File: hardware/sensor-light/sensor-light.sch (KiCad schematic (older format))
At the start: 15 parts, among them J1 Power IN 12V, J2 PIR Sensor Header 2, J3 PIR Sensor Header 1, J4 PROG Header, J5 Light Sensor Header, J6 PWM Power OUT 12V, Q1 IRLML2502, SW1 Manual ON/OFF, U1 Reg 3.3V, U2 MSP430G2553IN20

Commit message: change lables on the schematic
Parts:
- J2: value PIR Sensor Header 2 -> PIR Sensor 2
- J3: value PIR Sensor Header 1 -> PIR Sensor 1
- J5: value Light Sensor Header -> Light Sensor
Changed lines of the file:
@@
 P 9650 4850
 F 0 "R2" V 9730 4850 50  0000 C CNN
-F 1 "100 KOhm" V 9650 4850 50  0000 C CNN
+F 1 "100 KOhm" V 9650 4850 50  0000 C BNN
 F 2 "" V 9580 4850 50  0001 C CNN
 F 3 "" H 9650 4850 50  0001 C CNN
@@
 P 9300 4200
 F 0 "R1" V 9380 4200 50  0000 C CNN
-F 1 "27 Ohm" V 9300 4200 50  0000 C CNN
+F 1 "27 Ohm" V 9300 4200 50  0000 C BNN
 F 2 "" V 9230 4200 50  0001 C CNN
 F 3 "" H 9300 4200 50  0001 C CNN
@@
 P 8950 3500
 F 0 "J5" H 8950 3775 50  0000 C CNN
-F 1 "Light Sensor Header" H 8975 3225 50  0000 C CNN
+F 1 "Light Sensor" H 8975 3225 50  0000 C CNN
 F 2 "" H 8950 3700 50  0001 C CNN
 F 3 "" H 8950 3700 50  0001 C CNN
@@
 P 3150 3950
 F 0 "J3" H 3150 4225 50  0000 C CNN
-F 1 "PIR Sensor Header 1" H 3175 3675 50  0000 C CNN
+F 1 "PIR Sensor 1" H 3175 3675 50  0000 C CNN
 F 2 "" H 3150 4150 50  0001 C CNN
 F 3 "" H 3150 4150 50  0001 C CNN
@@
 P 2550 4800
 F 0 "J2" H 2550 5075 50  0000 C CNN
-F 1 "PIR Sensor Header 2" H 2575 4525 50  0000 C CNN
+F 1 "PIR Sensor 2" H 2575 4525 50  0000 C CNN
 F 2 "" H 2550 5000 50  0001 C CNN
 F 3 "" H 2550 5000 50  0001 C CNN

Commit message: remove extra line on the schematics
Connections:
- wire segments 47 -> 62
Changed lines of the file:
@@
 $EndComp
 Wire Wire Line
-	1400 5500 9950 5500
+	1400 5500 1800 5500
+Wire Wire Line
+	1800 5500 2200 5500
+Wire Wire Line
+	2200 5500 2850 5500
+Wire Wire Line
+	2850 5500 3450 5500
+Wire Wire Line
+	3450 5500 3800 5500
+Wire Wire Line
+	3800 5500 5750 5500
+Wire Wire Line
+	5750 5500 7550 5500
+Wire Wire Line
+	7550 5500 7800 5500
+Wire Wire Line
+	7800 5500 8200 5500
+Wire Wire Line
+	8200 5500 8650 5500
+Wire Wire Line
+	8650 5500 9650 5500
+Wire Wire Line
+	9650 5500 9950 5500
 Wire Wire Line
 	5750 4950 5750 5500
 Wire Wire Line
-	2200 3300 8650 3300
+	2200 3300 2850 3300
+Wire Wire Line
+	2850 3300 3450 3300
+Wire Wire Line
+	3450 3300 5750 3300
+Wire Wire Line
+	5750 3300 6050 3300
+Wire Wire Line
+	6050 3300 8650 3300
 Wire Wire Line
 	5750 3300 5750 3600
@@
 Connection ~ 1800 5500
 Wire Wire Line
-	1400 2750 1400 5300
+	1400 2750 1400 3300
 Wire Wire Line
-	1400 3300 1950 3300
+	1400 3300 1400 5300
 Wire Wire Line
 	1400 2750 9950 2750

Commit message: first attempt to assign footprints and make a pcb
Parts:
- C1: footprint (none) -> Capacitors_THT:CP_Radial_D4.0mm_P2.00mm
- D1, D2: footprint (none) -> LEDs:LED_CREE-XQ_HandSoldering
- J1, J6: footprint (none) -> Socket_Strips:Socket_Strip_Straight_1x02_Pitch2.54mm
- J2, J3, J5: footprint (none) -> Socket_Strips:Socket_Strip_Straight_1x03_Pitch2.54mm
- J4: footprint (none) -> Socket_Strips:Socket_Strip_Straight_1x04_Pitch2.54mm
- Q1: footprint (none) -> TO_SOT_Packages_SMD:SOT-23_Handsoldering
- R1, R2: footprint (none) -> Resistors_SMD:R_1218_HandSoldering
- SW1: footprint (none) -> Buttons_Switches_THT:SW_PUSH_SMALL
- U2: footprint 20N -> Housings_DIP:DIP-20_W7.62mm_Socket
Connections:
- wire segments 62 -> 46
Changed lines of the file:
@@
 F 0 "U2" H 4250 4900 50  0000 C CNN
 F 1 "MSP430G2553IN20" H 7000 3750 50  0000 C CNN
-F 2 "20N" H 4300 3750 50  0001 C CIN
+F 2 "Housings_DIP:DIP-20_W7.62mm_Socket" H 4300 3750 50  0001 C CIN
 F 3 "" H 5700 4300 50  0001 C CNN
 	1    5750 4300
@@
 F 0 "C1" H 2225 4000 50  0000 L CNN
 F 1 "10uF" H 2225 3800 50  0000 L CNN
-F 2 "" H 2238 3750 50  0001 C CNN
+F 2 "Capacitors_THT:CP_Radial_D4.0mm_P2.00mm" H 2238 3750 50  0001 C CNN
 F 3 "" H 2200 3900 50  0001 C CNN
 	1    2200 3900
@@
 F 0 "R2" V 9730 4850 50  0000 C CNN
 F 1 "100 KOhm" V 9650 4850 50  0000 C BNN
-F 2 "" V 9580 4850 50  0001 C CNN
+F 2 "Resistors_SMD:R_1218_HandSoldering" V 9580 4850 50  0001 C CNN
 F 3 "" H 9650 4850 50  0001 C CNN
 	1    9650 4850
@@
 F 0 "R1" V 9380 4200 50  0000 C CNN
 F 1 "27 Ohm" V 9300 4200 50  0000 C BNN
-F 2 "" V 9230 4200 50  0001 C CNN
+F 2 "Resistors_SMD:R_1218_HandSoldering" V 9230 4200 50  0001 C CNN
 F 3 "" H 9300 4200 50  0001 C CNN
 	1    9300 4200
@@
 F 0 "J1" H 1100 5575 50  0000 C CNN
 F 1 "Power IN 12V" H 1100 5200 50  0000 C CNN
-F 2 "" H 1100 5500 50  0001 C CNN
+F 2 "Socket_Strips:Socket_Strip_Straight_1x02_Pitch2.54mm" H 1100 5500 50  0001 C CNN
 F 3 "" H 1100 5500 50  0001 C CNN
 	1    1100 5400
@@
 F 0 "J6" H 10050 3000 50  0000 C CNN
 F 1 "PWM Power OUT 12V" H 10150 2850 50  0000 C BNN
-F 2 "" H 10050 2850 50  0001 C CNN
+F 2 "Socket_Strips:Socket_Strip_Straight_1x02_Pitch2.54mm" H 10050 2850 50  0001 C CNN
 F 3 "" H 10050 2850 50  0001 C CNN
 	1    10050 2850
@@
 F 0 "Q1" H 10050 4250 50  0000 L CNN
 F 1 "IRLML2502" H 10050 4150 50  0000 L CNN
-F 2 "" H 10050 4300 50  0001 C CNN
+F 2 "TO_SOT_Packages_SMD:SOT-23_Handsoldering" H 10050 4300 50  0001 C CNN
 F 3 "" H 9850 4200 50  0001 C CNN
 	1    9850 4200
@@
 F 0 "J5" H 8950 3775 50  0000 C CNN
 F 1 "Light Sensor" H 8975 3225 50  0000 C CNN
-F 2 "" H 8950 3700 50  0001 C CNN
+F 2 "Socket_Strips:Socket_Strip_Straight_1x03_Pitch2.54mm" H 8950 3700 50  0001 C CNN
 F 3 "" H 8950 3700 50  0001 C CNN
 	1    8950 3500
@@
 F 0 "J3" H 3150 4225 50  0000 C CNN
 F 1 "PIR Sensor 1" H 3175 3675 50  0000 C CNN
-F 2 "" H 3150 4150 50  0001 C CNN
+F 2 "Socket_Strips:Socket_Strip_Straight_1x03_Pitch2.54mm" H 3150 4150 50  0001 C CNN
 F 3 "" H 3150 4150 50  0001 C CNN
 	1    3150 3950
@@
 F 0 "J2" H 2550 5075 50  0000 C CNN
 F 1 "PIR Sensor 2" H 2575 4525 50  0000 C CNN
-F 2 "" H 2550 5000 50  0001 C CNN
+F 2 "Socket_Strips:Socket_Strip_Straight_1x03_Pitch2.54mm" H 2550 5000 50  0001 C CNN
 F 3 "" H 2550 5000 50  0001 C CNN
 	1    2550 4800
@@
 F 0 "SW1" H 8200 5350 50  0000 C CNN
 F 1 "Manual ON/OFF" H 8200 5050 50  0000 C CNN
-F 2 "" H 8200 5200 50  0001 C CNN
+F 2 "Buttons_Switches_THT:SW_PUSH_SMALL" H 8200 5200 50  0001 C CNN
 F 3 "" H 8200 5200 50  0001 C CNN
 	1    8200 5200
@@
 F 0 "D2" H 7800 5150 50  0000 C CNN
 F 1 "Green" H 7800 4950 50  0000 C CNN
-F 2 "" H 7800 5050 50  0001 C CNN
+F 2 "LEDs:LED_CREE-XQ_HandSoldering" H 7800 5050 50  0001 C CNN
 F 3 "" H 7800 5050 50  0001 C CNN
 	1    7800 5050
@@
 F 0 "D1" H 7550 5350 50  0000 C CNN
 F 1 "Red" H 7550 5150 50  0000 C CNN
-F 2 "" H 7550 5250 50  0001 C CNN
+F 2 "LEDs:LED_CREE-XQ_HandSoldering" H 7550 5250 50  0001 C CNN
 F 3 "" H 7550 5250 50  0001 C CNN
 	1    7550 5250
@@
 F 0 "J4" H 5750 2575 50  0000 C CNN
 F 1 "PROG Header" H 5750 1800 50  0000 C CNN
-F 2 "" H 5750 2500 50  0001 C CNN
+F 2 "Socket_Strips:Socket_Strip_Straight_1x04_Pitch2.54mm" H 5750 2500 50  0001 C CNN
 F 3 "" H 5750 2500 50  0001 C CNN
 	1    5750 2200
@@
 $EndComp
 Wire Wire Line
-	1400 5500 1800 5500
-Wire Wire Line
-	1800 5500 2200 5500
-Wire Wire Line
-	2200 5500 2850 5500
-Wire Wire Line
-	2850 5500 3450 5500
-Wire Wire Line
-	3450 5500 3800 5500
-Wire Wire Line
-	3800 5500 5750 5500
-Wire Wire Line
-	5750 5500 7550 5500
-Wire Wire Line
-	7550 5500 7800 5500
-Wire Wire Line
-	7800 5500 8200 5500
-Wire Wire Line
-	8200 5500 8650 5500
-Wire Wire Line
-	8650 5500 9650 5500
-Wire Wire Line
-	9650 5500 9950 5500
+	1400 5500 9950 5500
 Wire Wire Line
 	5750 4950 5750 5500
 Wire Wire Line
-	2200 3300 2850 3300
-Wire Wire Line
-	2850 3300 3450 3300
-Wire Wire Line
-	3450 3300 5750 3300
-Wire Wire Line
-	5750 3300 6050 3300
-Wire Wire Line
-	6050 3300 8650 3300
+	2200 3300 8650 3300
 Wire Wire Line
 	5750 3300 5750 3600
@@
 Connection ~ 1800 5500
 Wire Wire Line
-	1400 2750 1400 3300
-Wire Wire Line
-	1400 3300 1400 5300
+	1400 2750 1400 5300
 Wire Wire Line
 	1400 2750 9950 2750

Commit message: add resistors to the indicator LEDs
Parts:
- added R3, R4: 56 Ohm, symbol R
- J1: symbol CONN_01X02_MALE -> CONN_01X02_MALE-RESCUE-sensor-light
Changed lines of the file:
@@
 EESchema Schematic File Version 2
+LIBS:sensor-light-rescue
 LIBS:power
 LIBS:device
@@
 $EndComp
 $Comp
-L CONN_01X02_MALE J1
+L CONN_01X02_MALE-RESCUE-sensor-light J1
 U 1 1 5A4A4E4F
 P 1100 5400
@@
 	0    1    1    0
 $EndComp
-Wire Wire Line
-	1400 5500 9950 5500
-Wire Wire Line
-	5750 4950 5750 5500
-Wire Wire Line
-	2200 3300 8650 3300
-Wire Wire Line
-	5750 3300 5750 3600
-Wire Wire Line
-	1800 3600 1800 5500
-Connection ~ 1800 5500
-Wire Wire Line
-	1400 2750 1400 5300
-Wire Wire Line
-	1400 2750 9950 2750
-Connection ~ 1400 3300
-Wire Wire Line
-	2200 3300 2200 3750
-Wire Wire Line
-	9950 2950 9950 4000
-Wire Wire Line
-	9950 5500 9950 4400
-Connection ~ 2200 5500
-Connection ~ 2200 3300
-Wire Wire Line
-	9650 4200 9650 4700
-Wire Wire Line
-	9650 5000 9650 5500
-Connection ~ 9650 5500
-Connection ~ 9650 4200
-Connection ~ 5750 5500
-Wire Wire Line
-	7450 4400 8400 4400
-Wire Wire Line
-	8400 4400 8400 3500
-Wire Wire Line
-	8400 3500 8650 3500
-Wire Wire Line
-	8650 3700 8650 5500
-Connection ~ 8650 5500
-Wire Wire Line
-	9450 4200 9650 4200
-Wire Wire Line
-	9150 4200 7450 4200
-Connection ~ 8200 5500
-Wire Wire Line
-	8200 4300 8200 4900
-Wire Wire Line
-	2850 5000 2850 5500
-Connection ~ 2850 5500
-Wire Wire Line
-	2850 4600 2850 3300
-Connection ~ 2850 3300
-Wire Wire Line
-	3450 3300 3450 3750
-Wire Wire Line
-	3450 5500 3450 4150
-Wire Wire Line
-	3450 3950 3600 3950
-Wire Wire Line
-	3600 3950 3600 4400
-Wire Wire Line
-	3600 4400 4050 4400
-Wire Wire Line
-	4050 4500 3150 4500
-Wire Wire Line
-	3150 4500 3150 4800
-Wire Wire Line
-	3150 4800 2850 4800
-Connection ~ 7550 5500
-Wire Wire Line
-	7800 5200 7800 5500
-Connection ~ 7800 5500
-Wire Wire Line
-	7550 5100 7550 4600
-Wire Wire Line
-	7550 4600 7450 4600
-Wire Wire Line
-	7800 4900 7800 4000
-Wire Wire Line
-	7800 4000 7450 4000
-Wire Wire Line
-	7450 4300 8200 4300
-Connection ~ 5750 3300
-Connection ~ 3450 3300
-Connection ~ 3450 5500
-Wire Wire Line
-	2200 5500 2200 4050
-Wire Wire Line
-	5450 2500 3800 2500
-Wire Wire Line
-	3800 2500 3800 5500
-Connection ~ 3800 5500
-Wire Wire Line
-	4050 3850 4050 3100
-Wire Wire Line
-	4050 3100 5650 3100
-Wire Wire Line
-	5650 3100 5650 2500
-Wire Wire Line
-	7450 3850 7450 3100
-Wire Wire Line
-	7450 3100 5850 3100
-Wire Wire Line
-	5850 3100 5850 2500
-Wire Wire Line
-	7550 5500 7550 5400
-Wire Wire Line
-	6050 2500 6050 3300
-Connection ~ 6050 3300
 NoConn ~ 7450 4100
 NoConn ~ 7450 4500
@@
 NoConn ~ 4050 4600
 NoConn ~ 4050 4700
+$Comp
+L R R3
+U 1 1 5A4C95F9
+P 7550 4950
+F 0 "R3" V 7630 4950 50  0000 C CNN
+F 1 "56 Ohm" V 7550 4950 50  0000 C CNN
+F 2 "" V 7480 4950 50  0001 C CNN
+F 3 "" H 7550 4950 50  0001 C CNN
+	1    7550 4950
+	1    0    0    -1
+$EndComp
+$Comp
+L R R4
+U 1 1 5A4C9666
+P 7800 4750
+F 0 "R4" V 7880 4750 50  0000 C CNN
+F 1 "56 Ohm" V 7800 4750 50  0000 C CNN
+F 2 "" V 7730 4750 50  0001 C CNN
+F 3 "" H 7800 4750 50  0001 C CNN
+	1    7800 4750
+	1    0    0    -1
+$EndComp
+Wire Wire Line
+	1400 5500 9950 5500
+Wire Wire Line
+	5750 4950 5750 5500
+Wire Wire Line
+	2200 3300 8650 3300
+Wire Wire Line
+	5750 3300 5750 3600
+Wire Wire Line
+	1800 3600 1800 5500
+Connection ~ 1800 5500
+Wire Wire Line
+	1400 2750 1400 5300
+Wire Wire Line
+	1400 2750 9950 2750
+Connection ~ 1400 3300
+Wire Wire Line
+	2200 3300 2200 3750
+Wire Wire Line
+	9950 2950 9950 4000
+Wire Wire Line
+	9950 5500 9950 4400
+Connection ~ 2200 5500
+Connection ~ 2200 3300
+Wire Wire Line
+	9650 4200 9650 4700
+Wire Wire Line
+	9650 5000 9650 5500
+Connection ~ 9650 5500
+Connection ~ 9650 4200
+Connection ~ 5750 5500
+Wire Wire Line
+	7450 4400 8400 4400
+Wire Wire Line
+	8400 4400 8400 3500
+Wire Wire Line
+	8400 3500 8650 3500
+Wire Wire Line
+	8650 3700 8650 5500
+Connection ~ 8650 5500
+Wire Wire Line
+	9450 4200 9650 4200
+Wire Wire Line
+	9150 4200 7450 4200
+Connection ~ 8200 5500
+Wire Wire Line
+	8200 4300 8200 4900
+Wire Wire Line
+	2850 5000 2850 5500
+Connection ~ 2850 5500
+Wire Wire Line
+	2850 4600 2850 3300
+Connection ~ 2850 3300
+Wire Wire Line
+	3450 3300 3450 3750
+Wire Wire Line
+	3450 5500 3450 4150
+Wire Wire Line
+	3450 3950 3600 3950
+Wire Wire Line
+	3600 3950 3600 4400
+Wire Wire Line
+	3600 4400 4050 4400
+Wire Wire Line
+	4050 4500 3150 4500
+Wire Wire Line
+	3150 4500 3150 4800
+Wire Wire Line
+	3150 4800 2850 4800
+Connection ~ 7550 5500
+Wire Wire Line
+	7800 5200 7800 5500
+Connection ~ 7800 5500
+Wire Wire Line
+	7550 4600 7450 4600
+Wire Wire Line
+	7800 4000 7450 4000
+Wire Wire Line
+	7450 4300 8200 4300
+Connection ~ 5750 3300
+Connection ~ 3450 3300
+Connection ~ 3450 5500
+Wire Wire Line
+	2200 5500 2200 4050
+Wire Wire Line
+	5450 2500 3800 2500
+Wire Wire Line
+	3800 2500 3800 5500
+Connection ~ 3800 5500
+Wire Wire Line
+	4050 3850 4050 3100
+Wire Wire Line
+	4050 3100 5650 3100
+Wire Wire Line
+	5650 3100 5650 2500
+Wire Wire Line
+	7450 3850 7450 3100
+Wire Wire Line
+	7450 3100 5850 3100
+Wire Wire Line
+	5850 3100 5850 2500
+Wire Wire Line
+	7550 5500 7550 5400
+Wire Wire Line
+	6050 2500 6050 3300
+Connection ~ 6050 3300
+Wire Wire Line
+	7800 4600 7800 4000
+Wire Wire Line
+	7550 4800 7550 4600
 $EndSCHEMATC

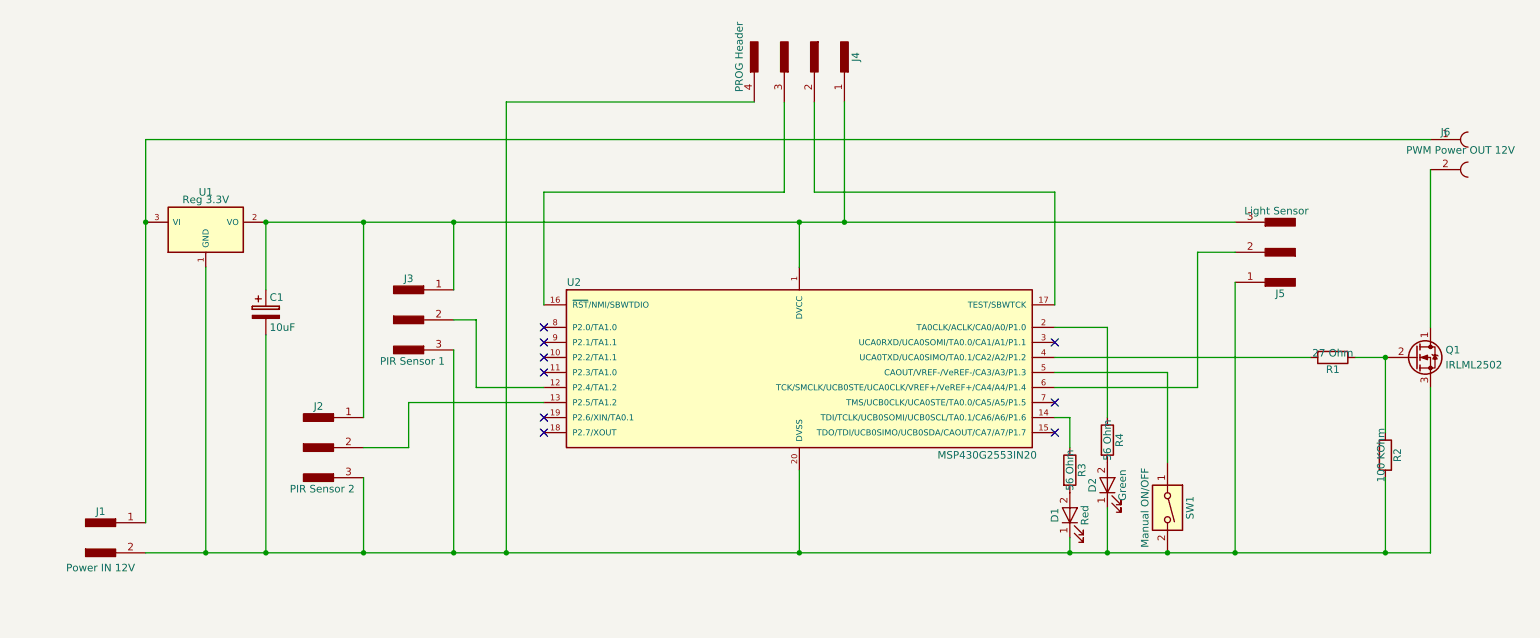
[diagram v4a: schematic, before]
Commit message: attempt to place components on the PCB
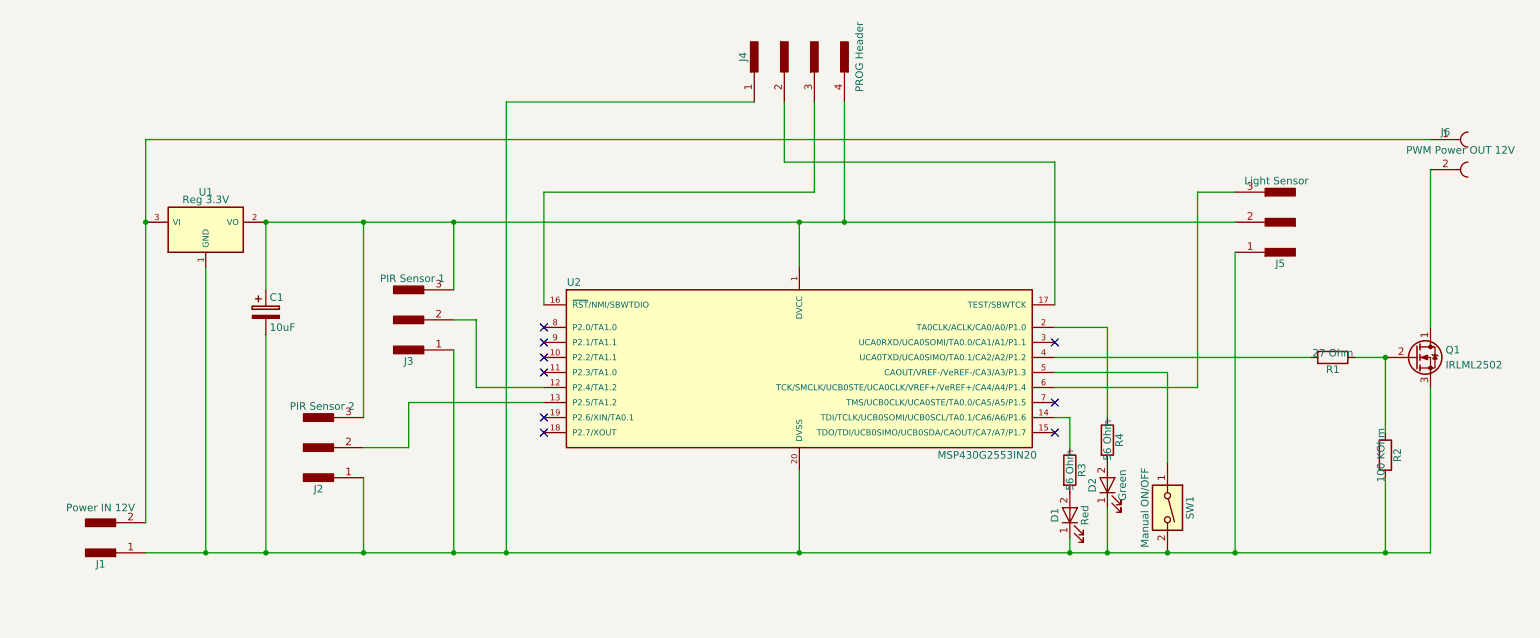
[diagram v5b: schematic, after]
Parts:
- C1: footprint Capacitors_THT:CP_Radial_D4.0mm_P2.00mm -> Capacitors_THT:CP_Radial_D5.0mm_P2.50mm
- D1, D2: footprint LEDs:LED_CREE-XQ_HandSoldering -> LEDs:LED_D3.0mm
- J1, J6: footprint Socket_Strips:Socket_Strip_Straight_1x02_Pitch2.54mm -> Connectors:AK300-2
- R1, R2: footprint Resistors_SMD:R_1218_HandSoldering -> Resistors_THT:R_Axial_DIN0411_L9.9mm_D3.6mm_P12.70mm_Horizontal
- R3, R4: footprint (none) -> Resistors_THT:R_Axial_DIN0411_L9.9mm_D3.6mm_P12.70mm_Horizontal
- SW1: footprint Buttons_Switches_THT:SW_PUSH_SMALL -> Buttons_Switches_THT:SW_PUSH_6mm_h5mm
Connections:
- net at C1.2, D1.1 (K), D2.1 (K)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: now also J1.1, J2.1, J3.1, J4.1; no longer J1.2, J2.3, J3.3, J4.4
- net at J5.2: now also C1.1, J2.3, J3.3, J4.4, U1.2 (VO), U2.1 (DVCC); no longer U2.6 (TCK/SMCLK/UCB0STE/UCA0CLK/VREF+/VeREF+/CA4/A4/P1.4)
- net at J6.1, U1.3 (VI): now also J1.2; no longer J1.1
- new net: J5.3, U2.6 (TCK/SMCLK/UCB0STE/UCA0CLK/VREF+/VeREF+/CA4/A4/P1.4)
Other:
- moved on the sheet: J5
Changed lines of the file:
@@
 F 0 "C1" H 2225 4000 50  0000 L CNN
 F 1 "10uF" H 2225 3800 50  0000 L CNN
-F 2 "Capacitors_THT:CP_Radial_D4.0mm_P2.00mm" H 2238 3750 50  0001 C CNN
+F 2 "Capacitors_THT:CP_Radial_D5.0mm_P2.50mm" H 2238 3750 50  0001 C CNN
 F 3 "" H 2200 3900 50  0001 C CNN
 	1    2200 3900
@@
 F 0 "R2" V 9730 4850 50  0000 C CNN
 F 1 "100 KOhm" V 9650 4850 50  0000 C BNN
-F 2 "Resistors_SMD:R_1218_HandSoldering" V 9580 4850 50  0001 C CNN
+F 2 "Resistors_THT:R_Axial_DIN0411_L9.9mm_D3.6mm_P12.70mm_Horizontal" V 9580 4850 50  0001 C CNN
 F 3 "" H 9650 4850 50  0001 C CNN
 	1    9650 4850
@@
 F 0 "R1" V 9380 4200 50  0000 C CNN
 F 1 "27 Ohm" V 9300 4200 50  0000 C BNN
-F 2 "Resistors_SMD:R_1218_HandSoldering" V 9230 4200 50  0001 C CNN
+F 2 "Resistors_THT:R_Axial_DIN0411_L9.9mm_D3.6mm_P12.70mm_Horizontal" V 9230 4200 50  0001 C CNN
 F 3 "" H 9300 4200 50  0001 C CNN
 	1    9300 4200
@@
 F 0 "J1" H 1100 5575 50  0000 C CNN
 F 1 "Power IN 12V" H 1100 5200 50  0000 C CNN
-F 2 "Socket_Strips:Socket_Strip_Straight_1x02_Pitch2.54mm" H 1100 5500 50  0001 C CNN
+F 2 "Connectors:AK300-2" H 1100 5500 50  0001 C CNN
 F 3 "" H 1100 5500 50  0001 C CNN
 	1    1100 5400
-	1    0    0    -1
+	1    0    0    1
 $EndComp
 $Comp
@@
 F 0 "J6" H 10050 3000 50  0000 C CNN
 F 1 "PWM Power OUT 12V" H 10150 2850 50  0000 C BNN
-F 2 "Socket_Strips:Socket_Strip_Straight_1x02_Pitch2.54mm" H 10050 2850 50  0001 C CNN
+F 2 "Connectors:AK300-2" H 10050 2850 50  0001 C CNN
 F 3 "" H 10050 2850 50  0001 C CNN
 	1    10050 2850
@@
 L CONN_01X03_MALE J5
 U 1 1 5A4A4FE3
-P 8950 3500
-F 0 "J5" H 8950 3775 50  0000 C CNN
-F 1 "Light Sensor" H 8975 3225 50  0000 C CNN
-F 2 "Socket_Strips:Socket_Strip_Straight_1x03_Pitch2.54mm" H 8950 3700 50  0001 C CNN
-F 3 "" H 8950 3700 50  0001 C CNN
-	1    8950 3500
+P 8950 3300
+F 0 "J5" H 8950 3575 50  0000 C CNN
+F 1 "Light Sensor" H 8975 3025 50  0000 C CNN
+F 2 "Socket_Strips:Socket_Strip_Straight_1x03_Pitch2.54mm" H 8950 3500 50  0001 C CNN
+F 3 "" H 8950 3500 50  0001 C CNN
+	1    8950 3300
 	-1   0    0    1
 $EndComp
@@
 F 3 "" H 3150 4150 50  0001 C CNN
 	1    3150 3950
-	1    0    0    -1
+	1    0    0    1
 $EndComp
 $Comp
@@
 F 3 "" H 2550 5000 50  0001 C CNN
 	1    2550 4800
-	1    0    0    -1
+	1    0    0    1
 $EndComp
 $Comp
@@
 F 0 "SW1" H 8200 5350 50  0000 C CNN
 F 1 "Manual ON/OFF" H 8200 5050 50  0000 C CNN
-F 2 "Buttons_Switches_THT:SW_PUSH_SMALL" H 8200 5200 50  0001 C CNN
+F 2 "Buttons_Switches_THT:SW_PUSH_6mm_h5mm" H 8200 5200 50  0001 C CNN
 F 3 "" H 8200 5200 50  0001 C CNN
 	1    8200 5200
@@
 F 0 "D2" H 7800 5150 50  0000 C CNN
 F 1 "Green" H 7800 4950 50  0000 C CNN
-F 2 "LEDs:LED_CREE-XQ_HandSoldering" H 7800 5050 50  0001 C CNN
+F 2 "LEDs:LED_D3.0mm" H 7800 5050 50  0001 C CNN
 F 3 "" H 7800 5050 50  0001 C CNN
 	1    7800 5050
@@
 F 0 "D1" H 7550 5350 50  0000 C CNN
 F 1 "Red" H 7550 5150 50  0000 C CNN
-F 2 "LEDs:LED_CREE-XQ_HandSoldering" H 7550 5250 50  0001 C CNN
+F 2 "LEDs:LED_D3.0mm" H 7550 5250 50  0001 C CNN
 F 3 "" H 7550 5250 50  0001 C CNN
 	1    7550 5250
@@
 F 3 "" H 5750 2500 50  0001 C CNN
 	1    5750 2200
-	0    1    1    0
+	0    -1   1    0
 $EndComp
 NoConn ~ 7450 4100
@@
 F 0 "R3" V 7630 4950 50  0000 C CNN
 F 1 "56 Ohm" V 7550 4950 50  0000 C CNN
-F 2 "" V 7480 4950 50  0001 C CNN
+F 2 "Resistors_THT:R_Axial_DIN0411_L9.9mm_D3.6mm_P12.70mm_Horizontal" V 7480 4950 50  0001 C CNN
 F 3 "" H 7550 4950 50  0001 C CNN
 	1    7550 4950
@@
 F 0 "R4" V 7880 4750 50  0000 C CNN
 F 1 "56 Ohm" V 7800 4750 50  0000 C CNN
-F 2 "" V 7730 4750 50  0001 C CNN
+F 2 "Resistors_THT:R_Axial_DIN0411_L9.9mm_D3.6mm_P12.70mm_Horizontal" V 7730 4750 50  0001 C CNN
 F 3 "" H 7800 4750 50  0001 C CNN
 	1    7800 4750
@@
 	7450 4400 8400 4400
 Wire Wire Line
-	8400 4400 8400 3500
-Wire Wire Line
-	8400 3500 8650 3500
-Wire Wire Line
-	8650 3700 8650 5500
+	8400 4400 8400 3100
+Wire Wire Line
+	8400 3100 8650 3100
+Wire Wire Line
+	8650 3500 8650 5500
 Connection ~ 8650 5500
 Wire Wire Line
@@
 	4050 3850 4050 3100
 Wire Wire Line
-	4050 3100 5650 3100
-Wire Wire Line
-	5650 3100 5650 2500
-Wire Wire Line
-	7450 3850 7450 3100
-Wire Wire Line
-	7450 3100 5850 3100
+	4050 3100 5850 3100
 Wire Wire Line
 	5850 3100 5850 2500
 Wire Wire Line
+	7450 3850 7450 2900
+Wire Wire Line
+	7450 2900 5650 2900
+Wire Wire Line
+	5650 2900 5650 2500
+Wire Wire Line
 	7550 5500 7550 5400
